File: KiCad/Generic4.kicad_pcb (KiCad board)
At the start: 2 copper layers, 13.2 x 19.5 mm, 11 parts, among them J1 I/O, J2 SPOX, U1 ESP32-PICO-MINI-02, U2 LMR16006+FB

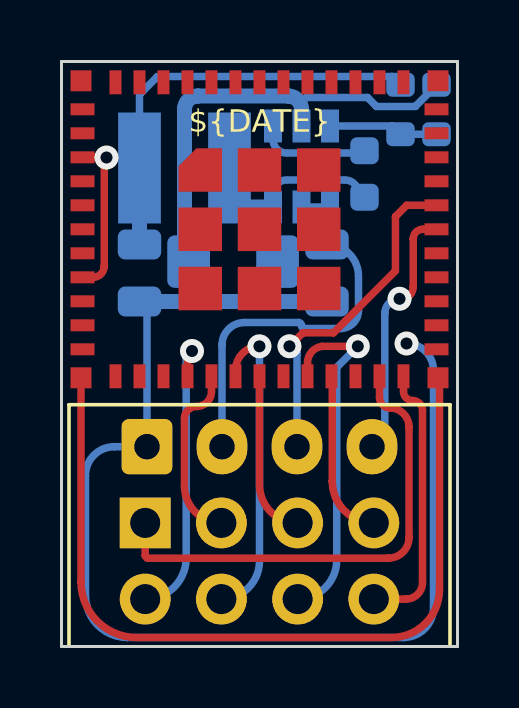
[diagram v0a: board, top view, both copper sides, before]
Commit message: Tidy
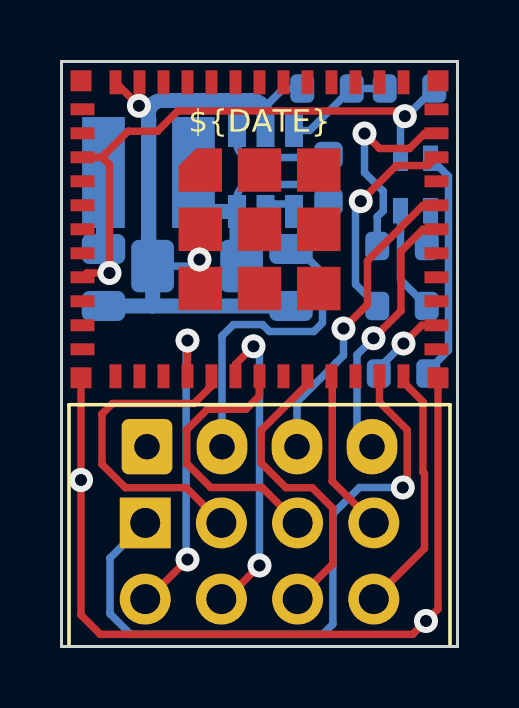
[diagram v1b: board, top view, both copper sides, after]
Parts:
- added D1: RGB, RevK:LED-RGB-1.6x1.6, B.Cu at (105.2, 42.7)
- added R1: 680R, RevK:R_0603, B.Cu at (104.8, 46.8)
- added R2: 2K, RevK:R_0603, B.Cu at (104.8, 44.8)
- added R3: 220R, RevK:R_0603, B.Cu at (104.8, 49.0)
- moved R5 3.72 mm to (102.2, 39.5), turned to 0 degrees
- moved U2 1.21 mm to (100.2, 42.2)
- moved R4 0.76 mm to (105.0, 39.5), turned to 180 degrees
- renumbered D1 to D2, R1 to R4, R2 to R5
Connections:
- U1 pad 26: unconnected-(U1-Pad26) -> B
- U1 pad 33: unconnected-(U1-Pad33) -> R
- U1 pad 34: unconnected-(U1-Pad34) -> G
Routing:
- net GND: track 67.1 -> 38.7 mm, vias 1 -> 4
- net Net-(D1-Pad4): track 0.00 -> 7.60 mm
- net R: track 0.00 -> 7.00 mm, vias 0 -> 1
- net G: track 0.00 -> 6.91 mm, vias 0 -> 1
- net GPIO0: track 16.2 -> 21.9 mm, vias 0 -> 1
- net IO2: track 6.02 -> 10.8 mm
- net IO4: track 5.56 -> 9.18 mm
- net Net-(D1-Pad2): track 0.00 -> 3.54 mm
- net B: track 0.00 -> 2.59 mm, vias 0 -> 1
- net EN: track 18.0 -> 20.1 mm, vias 1 -> 2
- net IO5: track 11.8 -> 10.1 mm, vias 1 -> 0
- net Net-(D1-Pad3): track 0.00 -> 1.23 mm
- net TX: track 11.4 -> 10.2 mm
- net DC: track 12.5 -> 11.5 mm
- net IO7: track 9.13 -> 8.42 mm
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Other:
- board text removed: "${DATE}"
